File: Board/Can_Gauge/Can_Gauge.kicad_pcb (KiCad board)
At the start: 2 copper layers, 46 x 46 mm, 33 parts, among them J1 FTDI-Port, J2 CAN, J3 LED 12V, J4 12V, J5 GND, M1 Stepper_Motor, U1 ATMEGA328P-AU, U2 MCP2515-xST, U3 MCP2551-I-SN, U4 L78L05_SOT89, Y1 16MHz, Y2 16MHz

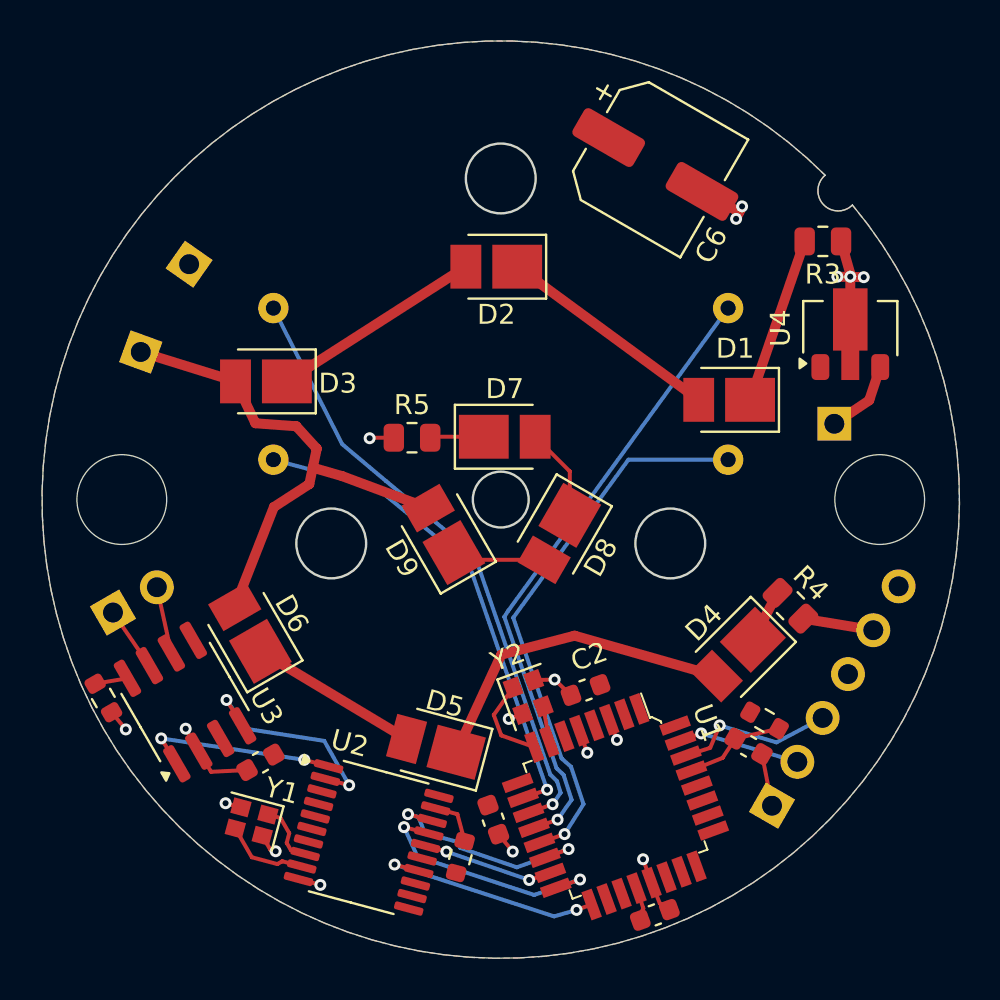
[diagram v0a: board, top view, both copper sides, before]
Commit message: Board adjustments
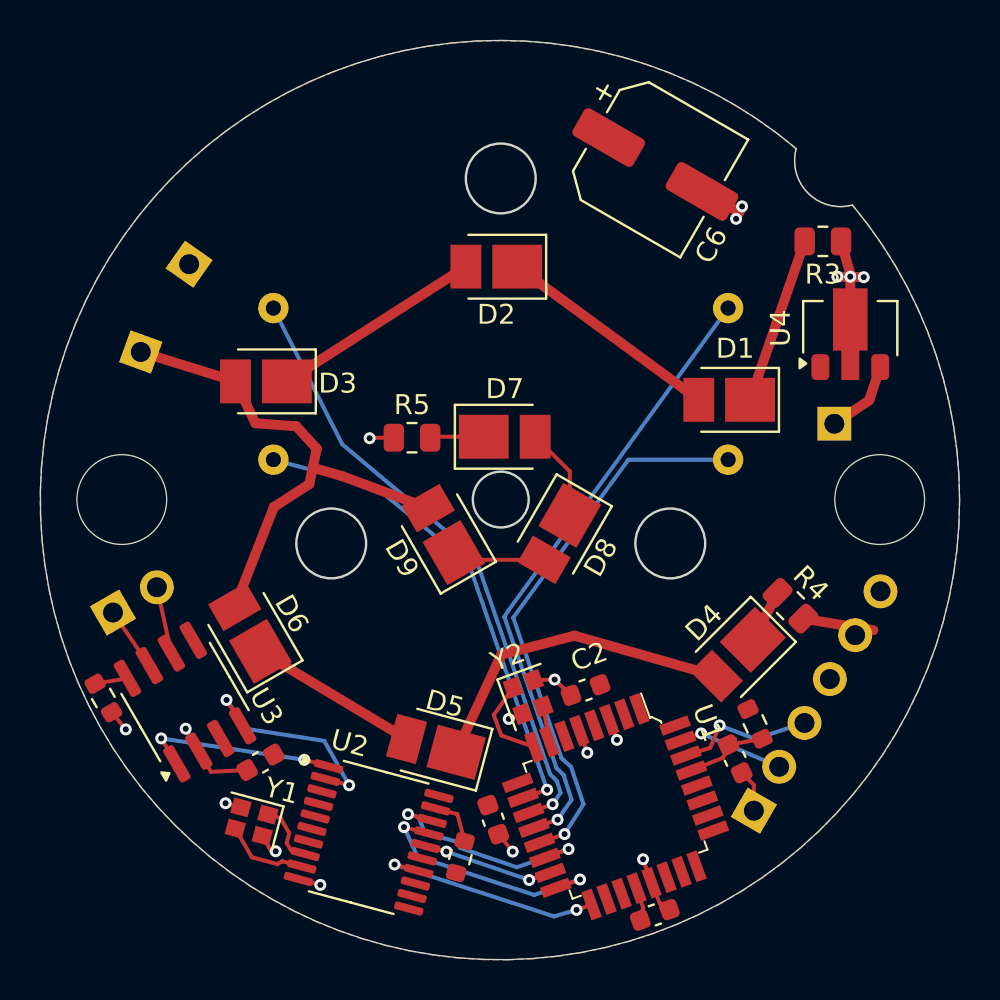
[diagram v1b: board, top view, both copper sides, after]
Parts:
- moved J1 0.94 mm to (162.7, 115.6)
- moved C3 0.92 mm to (161.8, 113.0), turned to 115.4 degrees
- moved R2 0.51 mm to (162.8, 111.2), turned to 115.4 degrees
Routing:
- net TX: track 8.09 -> 7.00 mm
- net RX: track 6.12 -> 5.35 mm
- net Net-(U1-PC6): track 5.08 -> 4.55 mm
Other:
- board size 46 x 46 mm -> 46.1 x 46.1 mm
- board text added: "12V"
- board text added: "12V LED"
- board text added: "CAN H L"
- board text added: "DTR RX TX 5V CTS G"
- board text added: "GND"
- board text added: "JoeM Can Gauge V0.2"
- board text removed: "DTR RX TX 5V CTX G"
- board text removed: "JoeM Can Gauge V0.1"
